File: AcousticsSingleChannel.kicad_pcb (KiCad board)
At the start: 4 copper layers, 25.4 x 44.1 mm, 59 parts, among them J1 87233-3, J2 87233-3, J3 87233-3, J8 22-05-3021, SW2 Switch_Omron_A6S-1104-PH_eec, U1 OPA1604AIPWR, U2 OPA1604AIPWR, U3 LTC6910-3CTS8#TRPBF, U4 LTC1197LIMS8#PBF

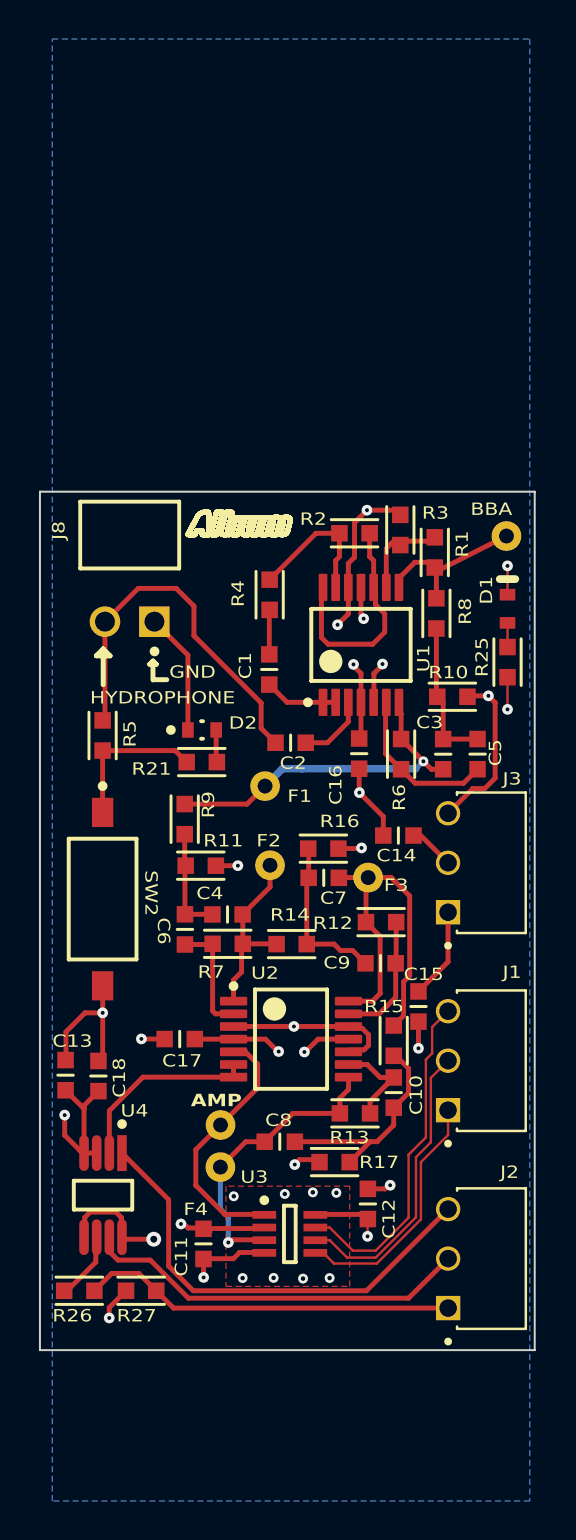
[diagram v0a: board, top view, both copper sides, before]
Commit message: Ready for review
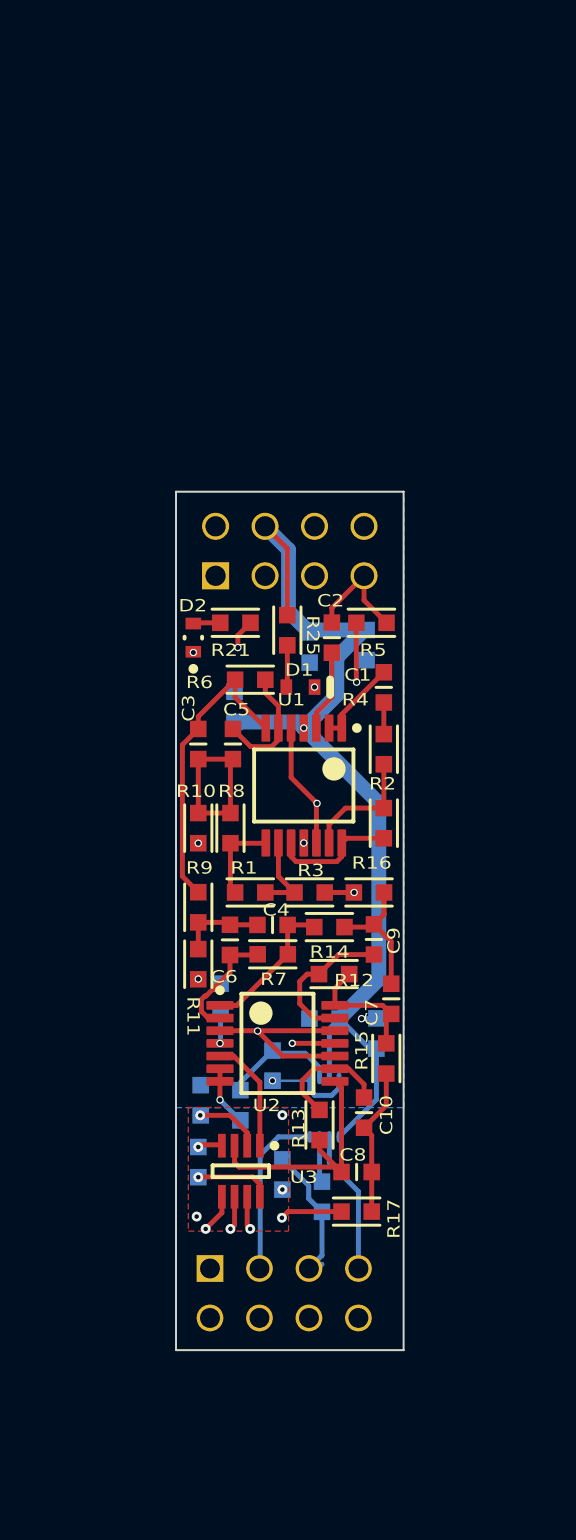
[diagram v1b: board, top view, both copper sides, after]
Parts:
- removed ? (x6): , AltiumImports:Probepoint
- removed G*** (x3): LOGO, LOGO
- removed J3: 87233-3, AltiumImports:TE_87233-3
- removed J8: 22-05-3021, AltiumImports:FP-22-05-3021-MFG
- removed SW2: Switch_Omron_A6S-1104-PH_eec, AltiumImports:Omron_A6S-1104-PH_0
- added C19: 1.5nF, AltiumImports:SMD-0603C, B.Cu at (147.5, 108.3)
- added R18: 25, AltiumImports:SMD-0603-RES, B.Cu at (145.8, 110.3)
- C11, C12, C13, C14, C15, C16, C17: moved to B.Cu
- C18: value 2.2µF -> 1µF; moved to B.Cu
- J1: value 87233-3 -> SSW-104-01-G-D; footprint AltiumImports:TE_87233-3 -> Accoustics:SAMTEC_SSW-104-01-G-D; moved to B.Cu
- J2: value 87233-3 -> TSW-104-07-F-D; footprint AltiumImports:TE_87233-3 -> Accoustics:SAMTEC_TSW-104-07-F-D; moved to B.Cu
- R26: value 750 -> 0; moved to B.Cu
- R27: value 1k -> 0; moved to B.Cu
- U4: value LTC1197LIMS8#PBF -> ADS7042IDCUR; footprint AltiumImports:FP-MS8-8-05-08-1660-IPC_A -> Accoustics:DCU0008A_L; moved to B.Cu
- moved J1 29.9 mm to (144.6, 83.1), turned to 180 degrees
- moved R1 19.9 mm to (146.3, 99.4), turned to -90 degrees
- moved C15 19.3 mm to (149.4, 86.8)
- moved R3 19.2 mm to (149.4, 99.4), turned to -90 degrees
- moved C13 16.1 mm to (152.8, 106.6)
- moved R8 15.3 mm to (145.3, 96.1), turned to 180 degrees
- moved R5 15.0 mm to (152.6, 85.5), turned to -90 degrees
- moved R2 15.0 mm to (153.2, 95.8), turned to 0 degrees
- moved R10 14.7 mm to (143.7, 96.1), turned to 180 degrees
- moved R26 13.4 mm to (150.0, 115.0), turned to 0 degrees
- moved C3 12.6 mm to (143.7, 91.7), turned to 180 degrees
- moved C5 12.6 mm to (145.5, 91.7), turned to 180 degrees
- moved U4 12.2 mm to (150.2, 110.4), turned to 90 degrees
- moved C18 12.0 mm to (150.2, 105.8), turned to 90 degrees
- moved R25 11.4 mm to (148.2, 85.9), turned to 180 degrees
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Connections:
- net Net-(U1A-IN_A+) renamed /BufferBiasAmp/BUF_IN
- C12 pad 2: VCC -> +3.3V
- C13 pad 1: VCC -> +3.3V
- C14 pad 2: VCC -> +3.3V
- C15 pad 2: VCC -> +3.3V
- C16 pad 2: VCC -> +3.3V
- C17 pad 2: VCC -> +3.3V
- C18 pad 1: VCC -> +3.3V
- C2 pad 1: /BufferBiasAmp/BBA_IN -> /Hydro+
- R21 pad 2: Net-(R21-Pad2) -> /Mode_Sel
- R25 pad 2: VCC -> +3.3V
- R26 pad 1: Net-(J2-Pad1) -> Net-(J2-Pad05)
- R26 pad 2: Net-(U4-ADC_DOUT) -> Net-(U4-SDO)
- R27 pad 2: Net-(J2-Pad1) -> Net-(J2-Pad05)
- R5 pad 1: /BufferBiasAmp/BBA_IN -> /Hydro+
- R5 pad 2: Net-(R21-Pad2) -> /Mode_Sel
- U1 pad 4: VCC -> +3.3V
- U2 pad 4: VCC -> +3.3V
- U3 pad 5: /OutputAmplifier/G0_out -> /G0_out
- U3 pad 6: /OutputAmplifier/G1_out -> /G1_out
- U3 pad 7: /OutputAmplifier/G2_out -> /G2_out
- U3 pad 8: VCC -> +3.3V
- U4 pad 1: Net-(U4-~{CS}) -> +3.3V
- U4 pad 2: /Sig_Out -> Net-(U4-SCLK)
- U4 pad 3: GND -> Net-(U4-SDO)
- U4 pad 4: GND -> Net-(U4-CS_N)
- U4 pad 5: VCC -> GND
- U4 pad 6: Net-(U4-ADC_DOUT) -> Net-(U4-AINP)
- U4 pad 7: Net-(U4-CLK) -> +3.3V
- U4 pad 8: VCC -> GND
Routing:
- net +3.3V: track 0.00 -> 83.8 mm, vias 0 -> 3
- net /Mode_Sel: track 0.00 -> 45.3 mm, vias 0 -> 2
- net /G2_out: track 0.00 -> 36.7 mm, vias 0 -> 1
- net /G1_out: track 0.00 -> 36.1 mm, vias 0 -> 1
- net /G0_out: track 0.00 -> 35.7 mm, vias 0 -> 1
- net VCC: track 29.7 -> 0.00 mm, vias 7 -> 0
- net GND: track 36.4 -> 9.25 mm, vias 9 -> 8
- net Net-(U4-~{CS}): track 23.4 -> 0.00 mm
- net Net-(U4-CLK): track 20.0 -> 0.00 mm
- net /BufferBiasAmp/BBA_IN: track 19.3 -> 0.00 mm
- net Net-(J2-Pad1): track 19.3 -> 0.00 mm
- net /OutputAmplifier/G2_out: track 17.4 -> 0.00 mm
- net /OutputAmplifier/G1_out: track 15.1 -> 0.00 mm
- net /OutputAmplifier/G0_out: track 12.8 -> 0.00 mm
- net /Band Pass Filter/F3_Out: track 19.1 -> 6.60 mm
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- added copper zone on B.Cu, net GND
- removed copper zone on B.Cu, net VCC
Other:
- board size 25.4 x 44.1 mm -> 11.7 x 44.1 mm
- board text removed: "AMP"
- board text removed: "Acoustics Single Channel PCB"
- board text removed: "BBA"
- board text removed: "F1"
- board text removed: "F2"
- board text removed: "F3"
- board text removed: "F4"
- board text removed: "GND"
- board text removed: "HYDROPHONE"
- board text removed: "v1.1.2"

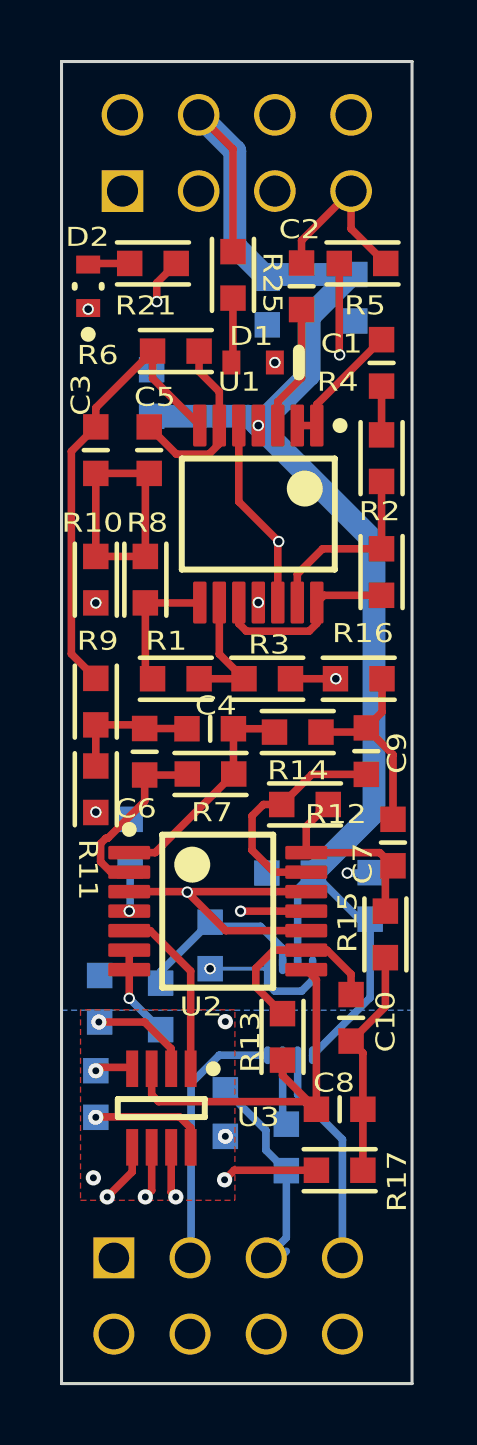
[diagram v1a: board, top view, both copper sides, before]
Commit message: Ready for Review.
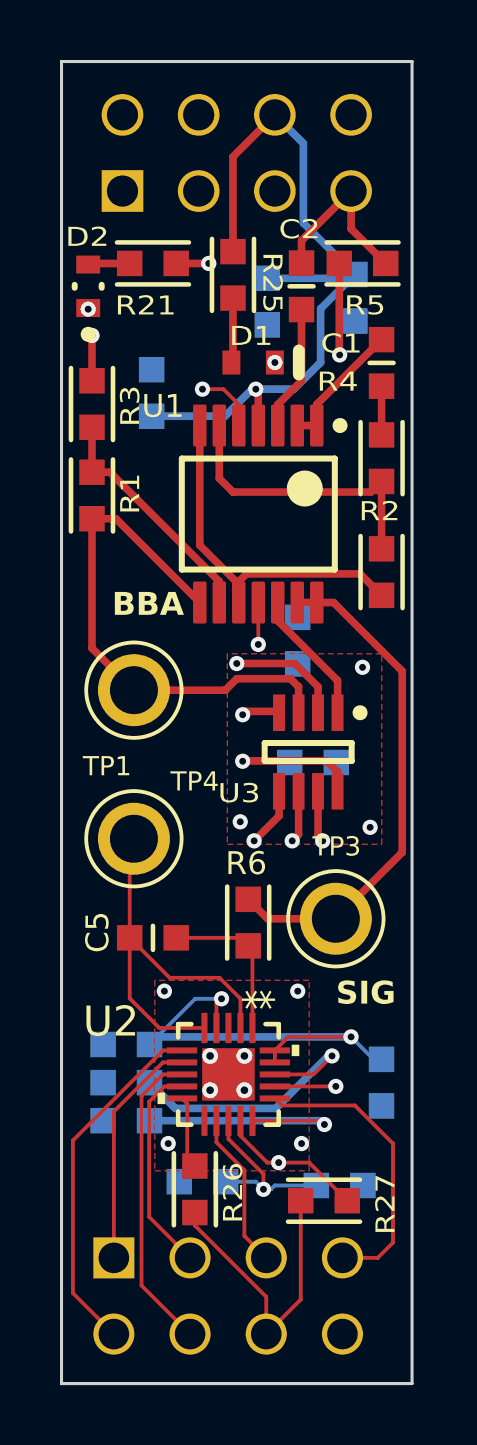
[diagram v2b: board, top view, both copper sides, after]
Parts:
- removed C10, C8, C9: 1000pF, AltiumImports:SMD-0603C
- removed C17: 1µF, AltiumImports:SMD-0603C
- removed C19: 1.5nF, AltiumImports:SMD-0603C
- removed R10: 698, AltiumImports:SMD-0603-RES
- removed R11: 536, AltiumImports:SMD-0603-RES
- removed R12: 165k, AltiumImports:SMD-0603-RES
- removed R13: 86.6k, AltiumImports:SMD-0603-RES
- removed R14: 11k, AltiumImports:SMD-0603-RES
- removed R15: 5.76k, AltiumImports:SMD-0603-RES
- removed R16: 332, AltiumImports:SMD-0603-RES
- removed R17: 174, AltiumImports:SMD-0603-RES
- removed R18: 25, AltiumImports:SMD-0603-RES
- removed R7: 41.2k, AltiumImports:SMD-0603-RES
- removed R8: 17.4k, AltiumImports:SMD-0603-RES
- removed R9: 13k, AltiumImports:SMD-0603-RES
- removed U4: ADS7042IDCUR, Accoustics:DCU0008A_L
- added TP1: 5005, Accoustics:KEYSTONE_5005, F.Cu at (144.9, 99.7)
- added TP3: 5005, Accoustics:KEYSTONE_5005, F.Cu at (151.7, 107.4)
- added TP4: 5006, Accoustics:KEYSTONE_5006, F.Cu at (144.9, 104.7)
- C13: value 1µF -> .1µF
- C3, C4, C6: value 1000pF -> 1µF; moved to B.Cu
- C5: value 1000pF -> 0F
- C7: value 1000pF -> .1µF; moved to B.Cu
- R26, R27: moved to F.Cu
- R6: value 54.9k -> 0
- U2: value OPA1604AIPWR -> ADS127L21IRUKT; footprint AltiumImports:PW0014A_N -> Accoustics:WQFN20_RUK_TEX
- moved C3 21.1 mm to (144.7, 112.8), turned to 90 degrees
- moved R6 19.2 mm to (148.8, 107.5), turned to 0 degrees
- moved C5 16.3 mm to (145.6, 108.0), turned to 90 degrees
- moved C6 14.5 mm to (147.2, 116.1), turned to -90 degrees
- moved C11 13.6 mm to (150.4, 98.1)
- moved C4 13.4 mm to (144.7, 114.1)
- moved C12 13.2 mm to (150.9, 102.2), turned to 90 degrees
- moved U3 12.8 mm to (150.8, 101.8)
- moved C7 11.6 mm to (151.8, 116.3), turned to 90 degrees
- moved R3 10.9 mm to (143.5, 90.2), turned to 0 degrees
- moved C18 7.90 mm to (144.7, 111.6)
- moved R1 6.72 mm to (143.5, 93.3), turned to 0 degrees
- moved C13 6.23 mm to (153.2, 112.8), turned to 180 degrees
- moved U2 5.45 mm to (148.1, 112.6), turned to -90 degrees
- moved R27 4.40 mm to (151.3, 116.8), turned to -90 degrees
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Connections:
- C12 pad 2: +3.3V -> +5V
- C13 pad 1: +3.3V -> +5V
- C14 pad 2: +3.3V -> +5V
- C15 pad 2: +3.3V -> +5V
- C16 pad 2: +3.3V -> +5V
- C18 pad 1: +3.3V -> +5V
- C3 pad 1: /Band Pass Filter/F1_In -> Net-(U2-CAPA)
- C3 pad 2: /Band Pass Filter/F1_Out -> GND
- C4 pad 1: /Band Pass Filter/F2_In -> Net-(U2-CAPD)
- C4 pad 2: /Band Pass Filter/F2_Out -> GND
- C5 pad 1: /Band Pass Filter/F1_In -> GND
- C5 pad 2: Net-(U1B-IN_B-) -> Net-(U2-AINP)
- C6 pad 1: /Band Pass Filter/F2_In -> GND
- C6 pad 2: Net-(U2A-IN_A-) -> +3.3V
- C7 pad 1: /Band Pass Filter/F3_In -> GND
- C7 pad 2: /Band Pass Filter/F3_Out -> +3.3V
- J2 pad 01: unconnected-(J2-Pad01) -> /CS
- J2 pad 02: unconnected-(J2-Pad02) -> /RESET
- J2 pad 03: Net-(U4-CS_N) -> /SCLK
- J2 pad 04: unconnected-(J2-Pad04) -> /SDI
- J2 pad 05: Net-(J2-Pad05) -> /CLK
- J2 pad 06: unconnected-(J2-Pad06) -> Net-(J2-Pad06)
- J2 pad 07: Net-(U4-SCLK) -> /START
- R2 pad 1: Net-(U1D-IN_D-) -> Net-(U1B-IN_B-)
- R25 pad 2: +3.3V -> +5V
- R26 pad 1: Net-(J2-Pad05) -> Net-(J2-Pad06)
- R26 pad 2: Net-(U4-SDO) -> /DOUT
- R27 pad 2: Net-(J2-Pad05) -> Net-(J2-Pad06)
- R4 pad 2: Net-(U1D-IN_D-) -> Net-(U1B-IN_B-)
- R6 pad 1: Net-(U1B-IN_B-) -> /Sig_Out
- R6 pad 2: /Band Pass Filter/F1_Out -> Net-(U2-AINP)
- U1 pad 12: AGND -> /OutputAmplifier/Amp_Out
- U1 pad 13: Net-(U1D-IN_D-) -> /Sig_Out
- U1 pad 14: /BufferBiasAmp/BBAmp_IN -> /Sig_Out
- U1 pad 4: +3.3V -> +5V
- U1 pad 7: /Band Pass Filter/F1_Out -> /BufferBiasAmp/BBAmp_IN
- U2 pad 1: /Band Pass Filter/F2_Out -> Net-(U2-AINP)
- U2 pad 10: AGND -> /DOUT
- U2 pad 11: GND -> unconnected-(U2-*DRDY-Pad11)
- U2 pad 12: AGND -> /CLK
- U2 pad 13: Net-(U2D-IN_D-) -> +3.3V
- U2 pad 14: /Band Pass Filter/F3_Out -> GND
- U2 pad 2: Net-(U2A-IN_A-) -> GND
- U2 pad 3: AGND -> unconnected-(U2-VCM-Pad3)
- U2 pad 4: +3.3V -> +5V
- U2 pad 5: /OutputAmplifier/Amp_Out -> GND
- U2 pad 6: /Sig_Out -> /RESET
- U2 pad 7: /Sig_Out -> /CS
- U2 pad 8: /Band Pass Filter/BPF_OUT -> /SDI
- U2 pad 9: Net-(U2C-IN_C-) -> /SCLK
- U3 pad 3: /Band Pass Filter/BPF_OUT -> /BufferBiasAmp/BBA_OUT
- U3 pad 8: +3.3V -> +5V
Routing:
- net +5V: track 0.00 -> 73.5 mm, vias 0 -> 4
- net +3.3V: track 83.8 -> 46.2 mm, vias 3 -> 1
- net AGND: track 25.3 -> 9.55 mm, vias 9 -> 10
- net /Band Pass Filter/F1_Out: track 15.5 -> 0.00 mm
- net GND: track 9.25 -> 23.5 mm, vias 8 -> 6
- net /Sig_Out: track 3.08 -> 16.8 mm, vias 1 -> 0
- net /Band Pass Filter/BPF_OUT: track 13.5 -> 0.00 mm
- net /BufferBiasAmp/BBA_OUT: track 4.47 -> 17.7 mm
- net /G2_out: track 36.7 -> 24.0 mm
- net /RESET: track 0.00 -> 11.9 mm
- net /G1_out: track 36.1 -> 24.7 mm
- net /SDI: track 0.00 -> 10.3 mm
- net /G0_out: track 35.7 -> 25.5 mm
- net Net-(J2-Pad06): track 0.00 -> 9.96 mm
- net /START: track 0.00 -> 9.76 mm
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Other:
- board text added: "BBA"
- board text added: "SIG"
